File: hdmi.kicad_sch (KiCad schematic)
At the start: 6 parts, among them J2101 FPC0.5-SMT-20P, U2101 RCLAMP0524P, U2102 RCLAMP0524P, U2103 RCLAMP0524P

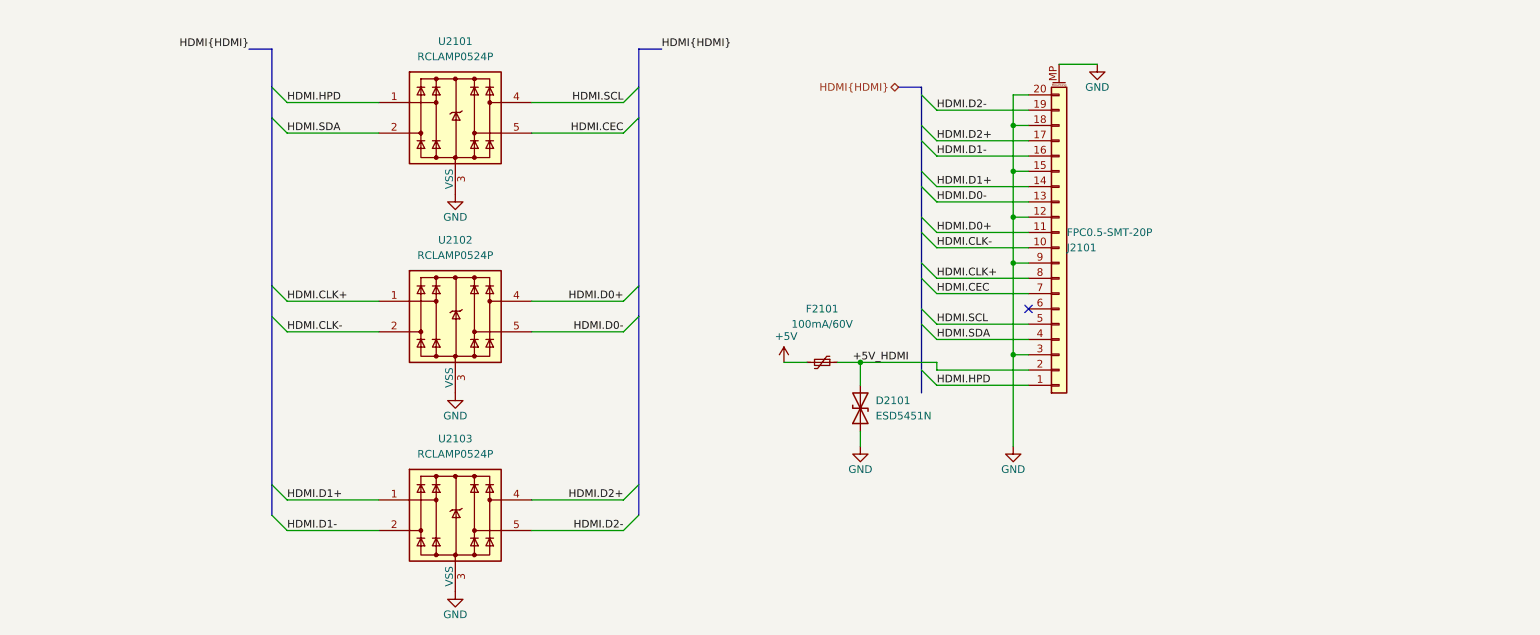
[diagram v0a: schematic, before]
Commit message: Further refinements
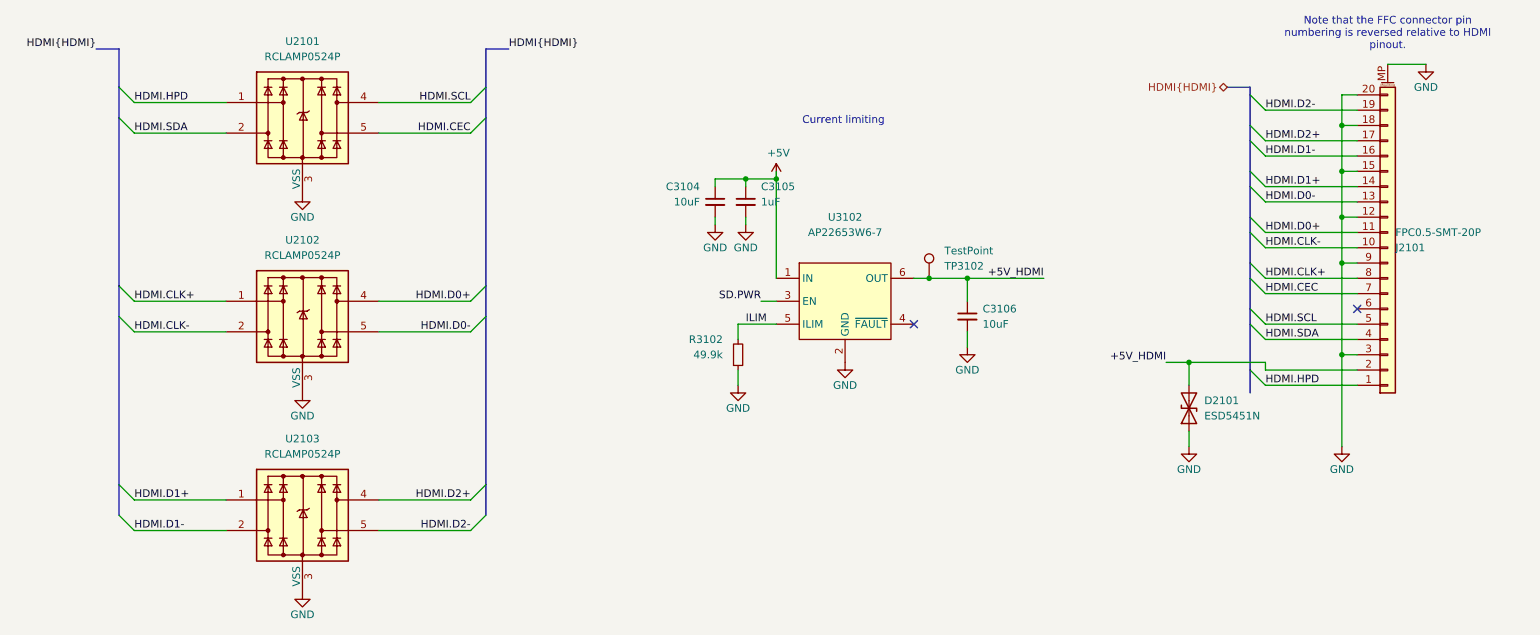
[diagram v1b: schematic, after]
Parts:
- removed F2101: 100mA/60V, Fuse:Fuse_1206_3216Metric, symbol Device:Polyfuse_Small
- added C3104, C3106: 10uF, Capacitor_SMD:C_0805_2012Metric, symbol Device:C_Small
- added C3105: 1uF, Capacitor_SMD:C_0402_1005Metric, symbol Device:C_Small
- added R3102: 49.9k, Resistor_SMD:R_0603_1608Metric, symbol Device:R_Small
- added TP3102: TestPoint, TestPoint:TestPoint_Pad_D1.0mm, symbol Connector:TestPoint
- added U3102: AP22653W6-7, Package_TO_SOT_SMD:SOT-23-6, symbol Hatlabs:AP22653
- J2101: LCSC C2914144 -> C11073
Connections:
- net +5V: now also C3104.1, C3105.1, U3102.1 (IN)
- net +5V_HDMI: now also C3106.1, TP3102.1, U3102.6 (OUT)
- net GND: now also C3104.2, C3105.2, C3106.2, R3102.1, U3102.2 (GND)
- new net ILIM: R3102.2, U3102.5 (ILIM)
- new net SD.PWR: U3102.3 (EN)
- no-connect marks 1 -> 2
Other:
- note added: "Current limiting"
- note added: "Note that the FFC connector pin numbering is reversed relative to HDMI pinout."
- moved on the sheet: D2101, J2101, U2101, U2102, U2103
